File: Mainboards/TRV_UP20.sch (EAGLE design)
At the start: 22 parts, among them IC2 MEGA328P-AU, IC3 LP2992-IM5-3.3, Q1 IRLML9301, X6 BU-SMA-V

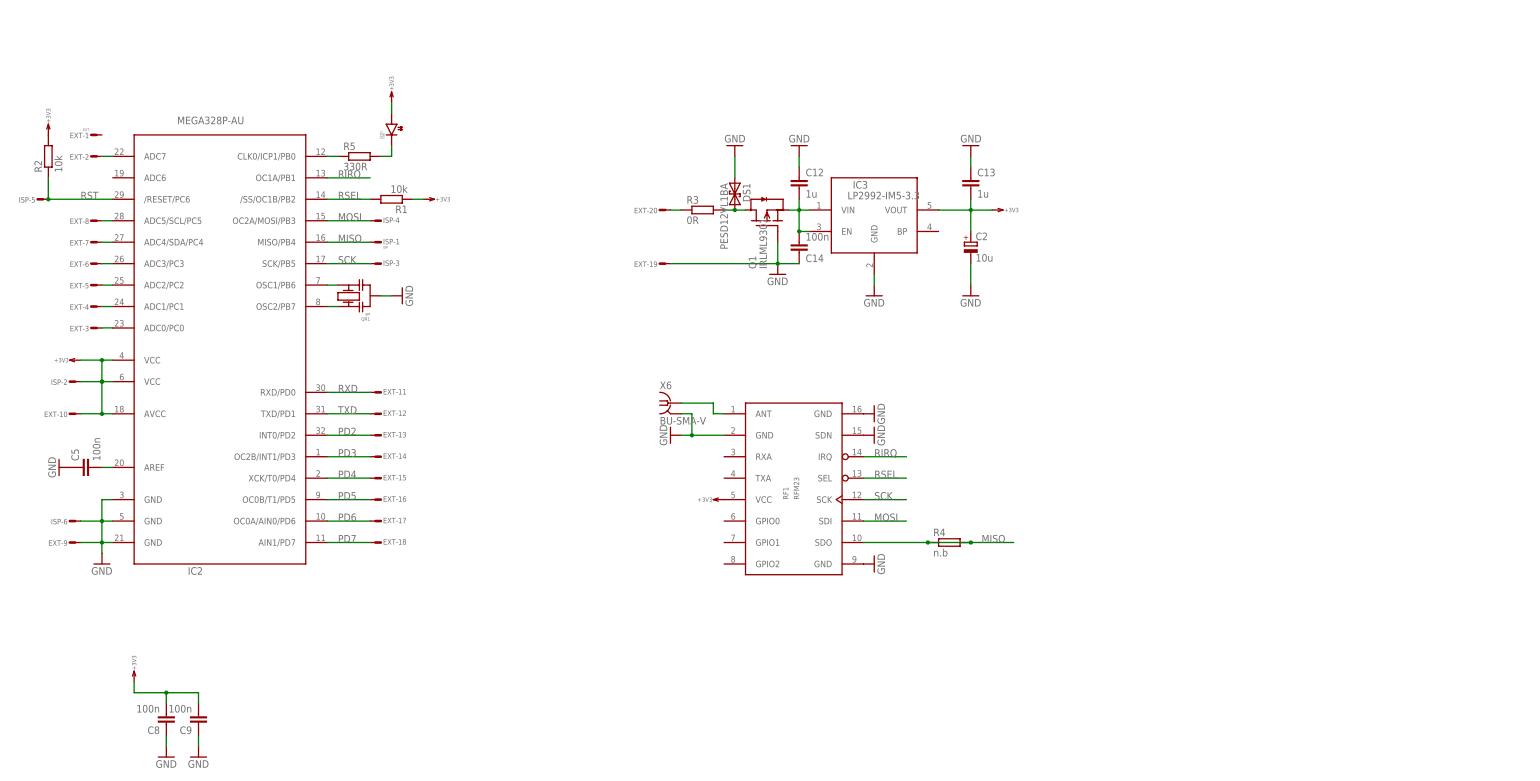
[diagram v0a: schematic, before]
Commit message: Reorganization
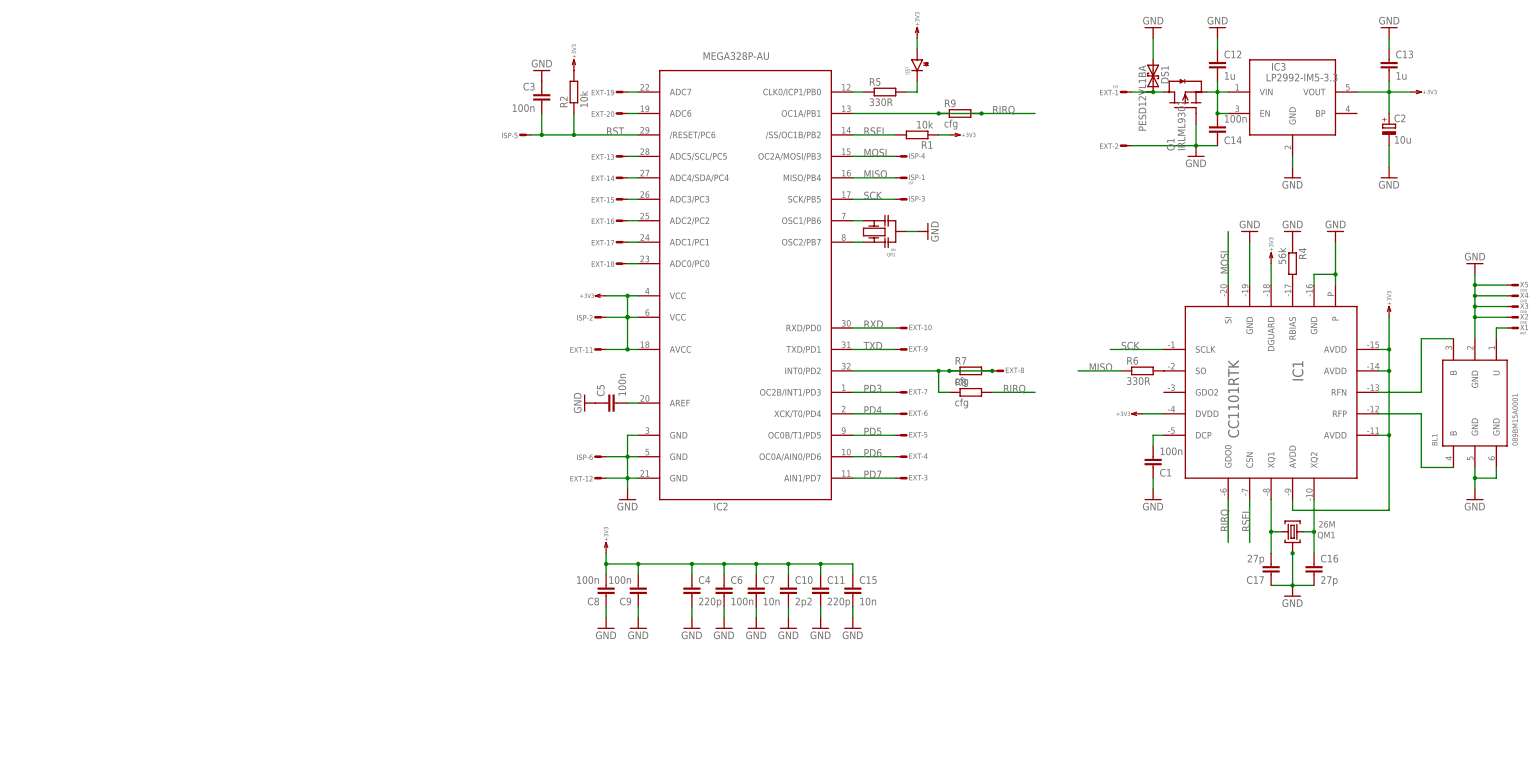
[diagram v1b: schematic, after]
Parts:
- removed R3: 0R, RCL:R0603
- removed RF1: RFM23, RF:RFM22S1
- removed X6: BU-SMA-V, Conn:BU-SMA-V
- added BL1: 089BM15A0001, RF:BL
- added C1, C6: 100n, RCL:C0402
- added C10: 2p2, RCL:C0402
- added C11, C4: 220p, RCL:C0402
- added C15, C7: 10n, RCL:C0402
- added C16, C17: 27p, RCL:C0402
- added C3: 100n, RCL:C0603
- added IC1: CC1101RTK, RF:CC110L
- added QM1: 26M, QUARTZ:QM3.2X2.5
- added R6: 330R, RCL:R0402
- added R7, R8, R9: cfg, RCL:R0402
- added X1: ANT, Conn:WIREPADS2.54/1.27
- added X2, X3, X4, X5: GND, Conn:WIREPADS2.54/1.27
- LED1: device Optic:LED0805 -> Optic:LEDT134
- QR1: device QUARTZ:QRCR -> QUARTZ:QRCE
- R1, R5: device RCL:R0603 -> RCL:R0402
- R4: value n.b -> 56k; device RCL:R0603 -> RCL:R0402
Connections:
- net LED renamed N$10
- removed net N$3: EXT-2.S, IC2.ADC7
- removed net N$9: EXT-20.S, R3.1
- removed net PD2: EXT-13.S, IC2.INT0/PD2
- new net ADC6: EXT-20.S, IC2.ADC6
- new net ADC7: EXT-19.S, IC2.ADC7
- new net N$11: EXT-8.S, IC2.INT0/PD2, R7.1, R7.2, R8.1
- new net N$13: BL1.B@3, IC1.RFN
- new net N$14: BL1.B@4, IC1.RFP
- new net N$16: BL1.U@1, X1.S
- new net N$17: C17.2, IC1.XQ1, QM1.2
- new net N$18: C16.1, IC1.XQ2, QM1.1
- new net N$2: IC1.RBIAS, R4.2
- new net N$4: IC1.SO, R6.2
- net +3V3: now also C10.1, C11.1, C15.1, C4.1, C6.1, C7.1, EXT-11.S, IC1.AVDD, IC1.AVDD@1, IC1.AVDD@2, IC1.AVDD@3, IC1.DGUARD, IC1.DVDD; no longer EXT-10.S, RF1.VCC
- net GND: now also BL1.GND@2, BL1.GND@5, BL1.GND@6, C1.1, C10.2, C11.2, C15.2, C16.2, C17.1, C3.1, C4.2, C6.2, C7.2, EXT-12.S, EXT-2.S, IC1.GND, IC1.GND@1, IC1.P, QM1.M1, QM1.M2, R4.1, X2.S, X3.S, X4.S, X5.S; no longer EXT-19.S, EXT-9.S, RF1.GND@16, RF1.GND@2, RF1.GND@9, RF1.SDN, X6G$1.GND
- net MISO: now also R6.1; no longer R4.1, R4.2, RF1.SDO
- net MOSI: now also IC1.SI; no longer RF1.SDI
- net N$1: now also C1.2, IC1.DCP; no longer RF1.ANT, X6G$1.1
- net N$5: now also EXT-1.S; no longer R3.2
- net PC0: now also EXT-18.S; no longer EXT-3.S
- net PC1: now also EXT-17.S; no longer EXT-4.S
- net PC2: now also EXT-16.S; no longer EXT-5.S
- net PC3: now also EXT-15.S; no longer EXT-6.S
- net PC4: now also EXT-14.S; no longer EXT-7.S
- net PC5: now also EXT-13.S; no longer EXT-8.S
- net PD3: now also EXT-7.S; no longer EXT-14.S
- net PD4: now also EXT-6.S; no longer EXT-15.S
- net PD5: now also EXT-5.S; no longer EXT-16.S
- net PD6: now also EXT-4.S; no longer EXT-17.S
- net PD7: now also EXT-3.S; no longer EXT-18.S
- net RIRQ: now also IC1.GDO0, R8.2, R9.1, R9.2; no longer RF1.IRQ
- net RSEL: now also IC1.CSN; no longer RF1.SEL
- net RST: now also C3.2
- net RXD: now also EXT-10.S; no longer EXT-11.S
- net SCK: now also IC1.SCLK; no longer RF1.SCK
- net TXD: now also EXT-9.S; no longer EXT-12.S
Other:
- note added: "UP20 868MHz"
- note added: "X13Home.org"
- note added: "comparator@gmx.de"
- moved on the sheet: C12, C13, C14, C2, C5, C8, C9, DS1, EXT-1, EXT-10, EXT-11, EXT-12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
